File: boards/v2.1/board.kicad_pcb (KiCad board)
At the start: 2 copper layers, 139.7 x 116.8 mm, 74 parts, among them J1 KF301-2P, J2 KF301-2P, J3 KF301-2P, J4 KF301-2P, J5 KF301-2P, J6 KF301-2P, J7 KF301-2P, K1 SRD-03VDC-SL-C, K2 SRD-03VDC-SL-C, K3 SRD-03VDC-SL-C, K4 SRD-03VDC-SL-C, P1 Pin Header, P2 Pin Header, P3 Pin Header, P4 Pin Header, P5 Pin Header, SW1 SS-12D00G 4mm, SW2 SS-12D00G 4mm, SW3 SS-12D00G 4mm, T1 ZMPT101B, T2 ZMPT101B, T3 ZMPT101B, U1 TP4056, U2 LM1117T-3.3

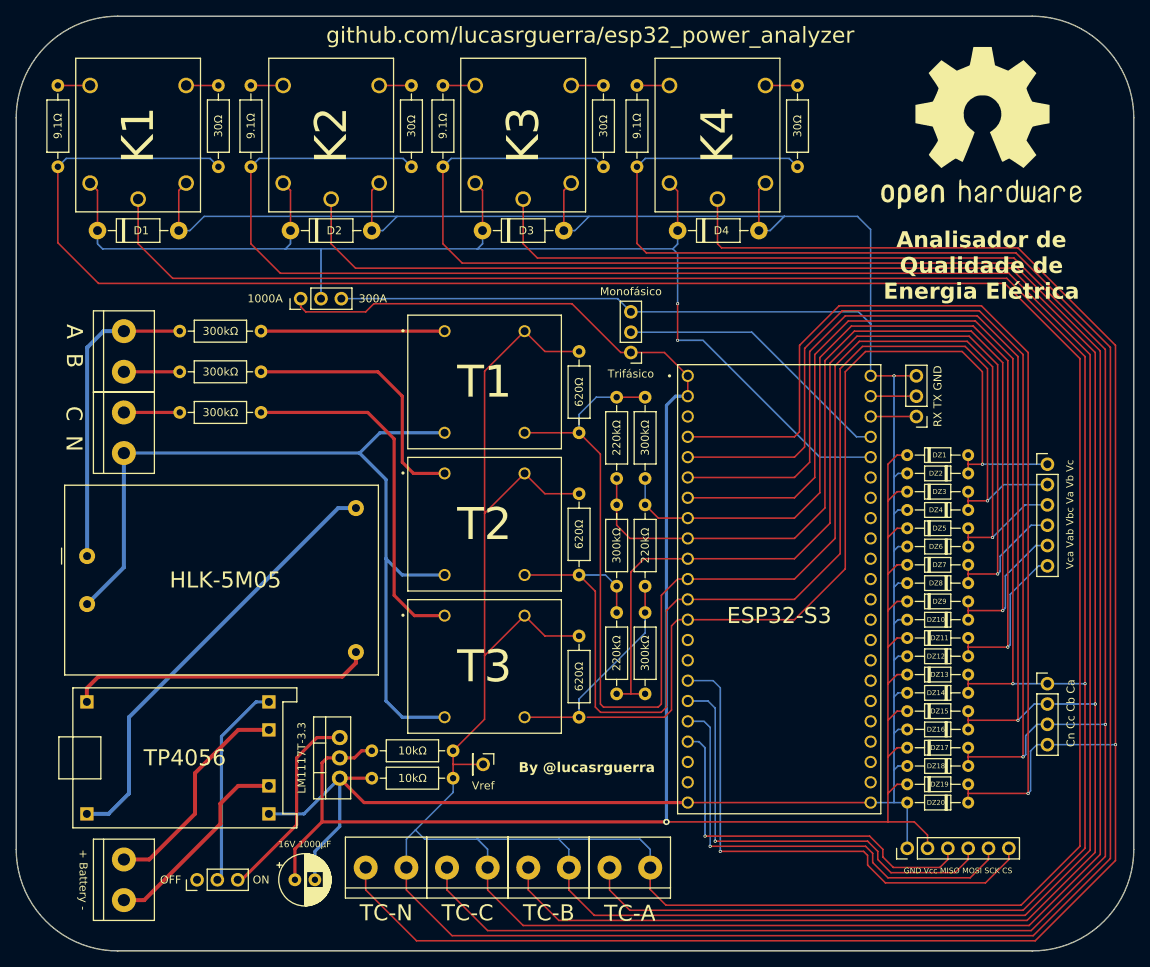
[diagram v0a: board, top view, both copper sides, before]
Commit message: Atualização da placa V2.1
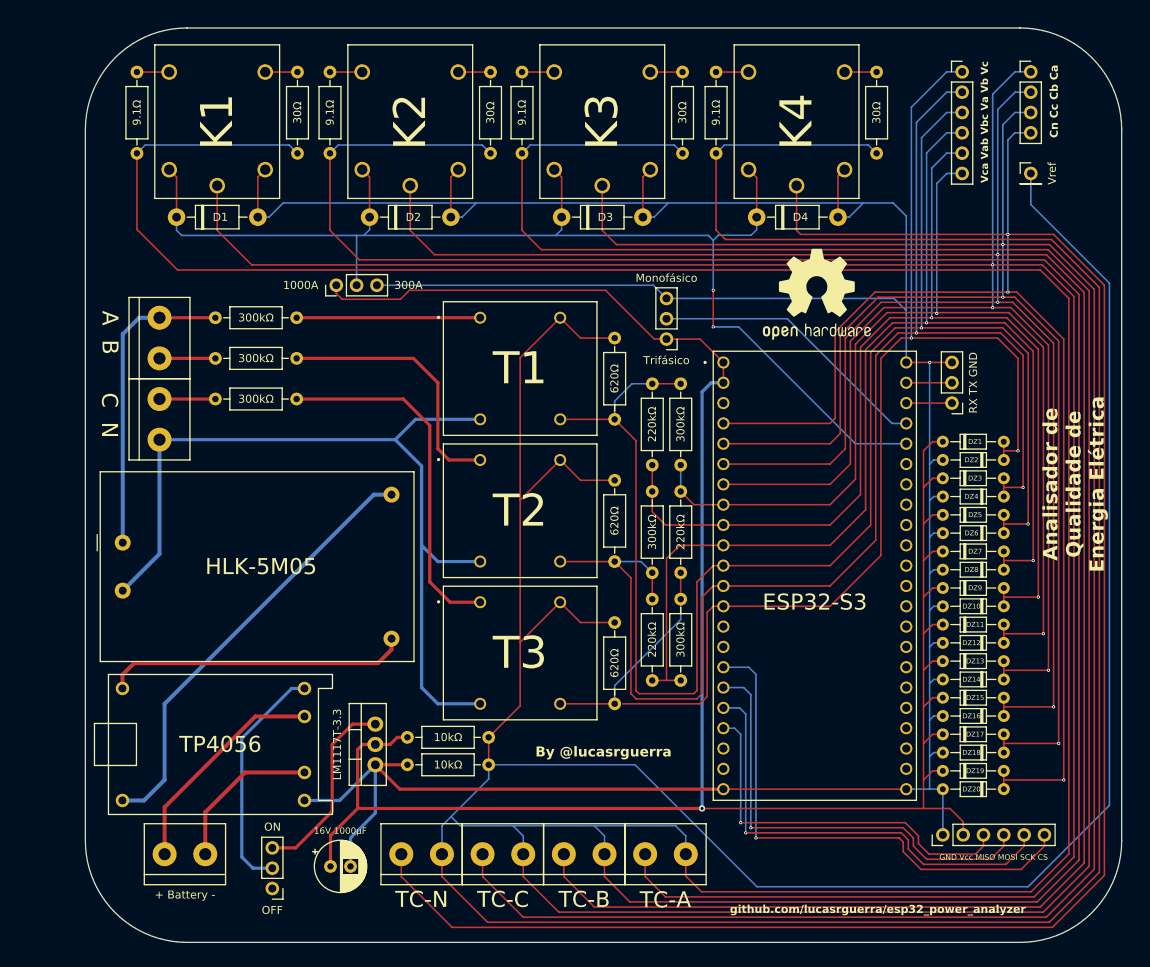
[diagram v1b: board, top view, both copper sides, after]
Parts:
- moved P2 100.7 mm to (203.9, 49.5), turned to 0 degrees
- moved P3 76.5 mm to (203.9, 36.8)
- moved P4 50.2 mm to (195.3, 36.8)
- moved G*** 29.3 mm to (177.2, 64.6)
- moved K2 10.0 mm to (126.3, 43.1)
- moved K3 10.0 mm to (150.3, 43.1)
- moved D1 10.0 mm to (97.1, 55.0)
- moved D2 10.0 mm to (121.3, 55.0)
- moved D3 10.0 mm to (145.3, 55.0)
- moved D4 10.0 mm to (169.6, 55.0)
- moved R16 10.0 mm to (116.3, 47.0)
- moved R17 10.0 mm to (140.3, 47.0)
- moved R18 10.0 mm to (164.6, 47.0)
- moved R19 10.0 mm to (112.2, 47.0)
- moved R20 10.0 mm to (136.4, 47.0)
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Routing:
- net TC A-1: track 1239.0 -> 1358.7 mm
- net C Vwave: track 140.6 -> 169.5 mm, vias 1 -> 2
- net B Vwave: track 152.3 -> 177.6 mm, vias 1 -> 2
- net A Vwave: track 178.5 -> 200.1 mm, vias 1 -> 2
- net BC Vwave: track 132.0 -> 148.9 mm, vias 1 -> 2
- net AB Vwave: track 126.8 -> 138.8 mm, vias 1 -> 2
- net A Cwave: track 376.0 -> 387.5 mm, vias 2 -> 3
- net CA Vwave: track 126.9 -> 133.9 mm, vias 1 -> 2
- net B Cwave: track 372.3 -> 379.0 mm, vias 2 -> 3
- net Battery -: track 25.5 -> 19.7 mm
- net N Cwave: track 367.6 -> 361.9 mm, vias 2 -> 3
- net GND: track 393.1 -> 387.7 mm
- net Vin: track 25.6 -> 29.6 mm
- net C Cwave: track 370.0 -> 370.6 mm, vias 2 -> 3
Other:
- board size 139.7 x 116.8 mm -> 129.5 x 114.3 mm
